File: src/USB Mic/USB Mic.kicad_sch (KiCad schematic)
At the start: 22 parts, among them IC1 ADUM3160BRWZ-RL, J1 GT-USB-7010ASV, Q1 LSK170B, U1 B0505S-3WR2_C7500927

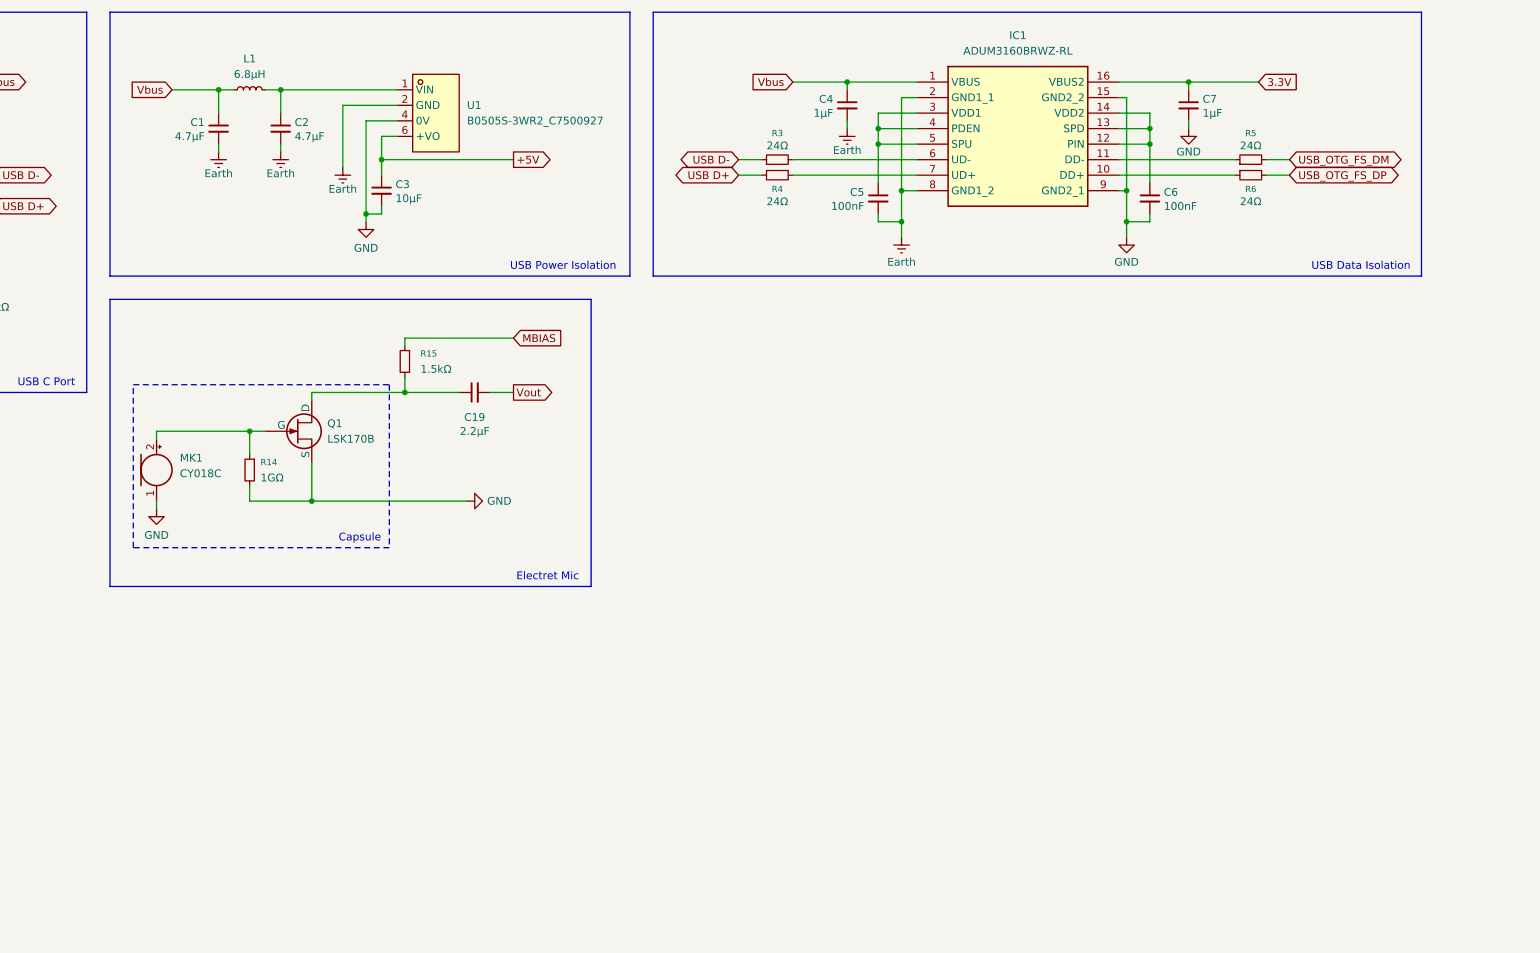
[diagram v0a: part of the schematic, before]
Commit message: Update to Rev. 5
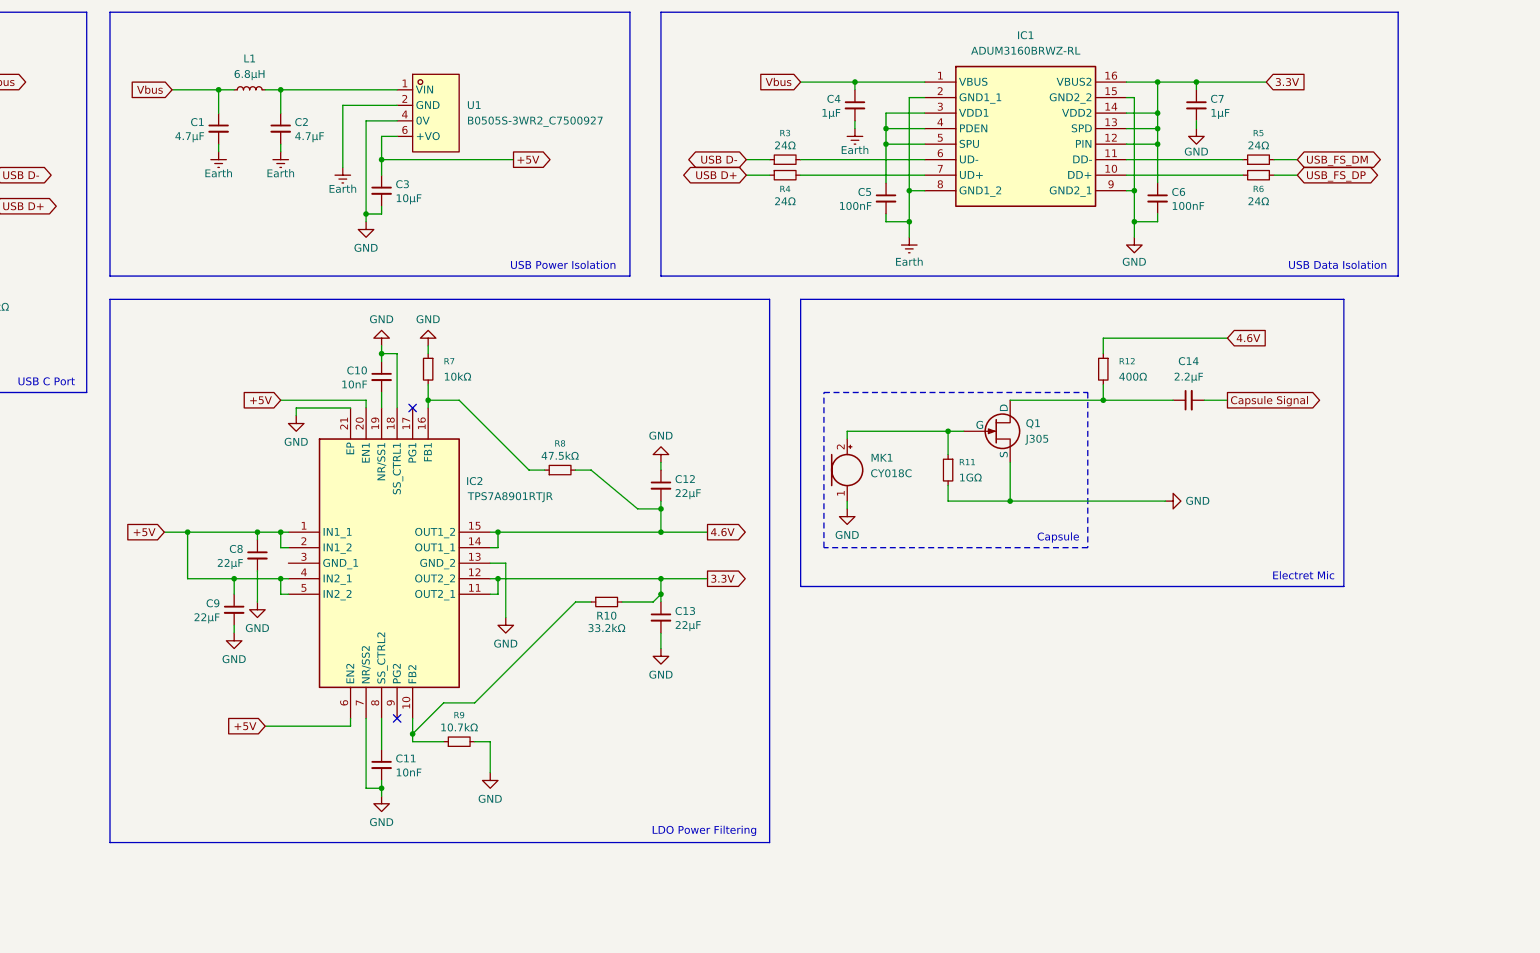
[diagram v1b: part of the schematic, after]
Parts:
- removed C19: 2.2µF, symbol Device:C_Small
- removed R14: 1GΩ, symbol Device:R_Small
- removed R15: 1.5kΩ, symbol Device:R_Small
- added C10, C11: 10nF, symbol Device:C_Small
- added C12, C13, C8, C9: 22µF, symbol Device:C_Small
- added C14: 2.2µF, symbol Device:C_Small
- added IC2: TPS7A8901RTJR, footprints:QFN50P400X400X80-21N-D, symbol TPS7A8901RTJR:TPS7A8901RTJR
- added R10: 33.2kΩ, symbol Device:R_Small
- added R11: 1GΩ, symbol Device:R_Small
- added R12: 400Ω, symbol Device:R_Small
- added R7: 10kΩ, symbol Device:R_Small
- added R8: 47.5kΩ, symbol Device:R_Small
- added R9: 10.7kΩ, symbol Device:R_Small
- Q1: value LSK170B -> J305
- U1: footprint easyeda2kicad:PWRM-TH_BXXXXS-3WR2 -> footprints:B0505S-3WR2
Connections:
- net +5V: now also C8.1, C9.1, IC2.1 (IN1_1), IC2.2 (IN1_2), IC2.20 (EN1), IC2.4 (IN2_1), IC2.5 (IN2_2), IC2.6 (EN2)
- net 3.3V: now also C6.1, IC1.12 (PIN), IC1.13 (SPD), IC1.14 (VDD2), C13.1, IC2.11 (OUT2_1), IC2.12 (OUT2_2), R10.2
- net GND: now also C10.1, C11.2, C12.1, C13.2, C8.2, C9.2, IC2.13 (GND_2), IC2.18 (SS_CTRL1), IC2.21 (EP), IC2.7 (NR/SS2), R11.2, R7.1, R9.2
- net at MK1.2 (+), Q1.2 (G): now also R11.1
- net at Q1.1 (D): now also C14.1, R12.2
- net USB_OTG_FS_DM renamed USB_FS_DM
- net USB_OTG_FS_DP renamed USB_FS_DP
- new net: IC2.10 (FB2), R10.1, R9.1
- new net: C10.2, IC2.19 (NR/SS1)
- new net: IC2.16 (FB1), R7.2, R8.1
- new net: C11.1, IC2.8 (SS_CTRL2)
- new net 4.6V: C12.2, IC2.14 (OUT1_1), IC2.15 (OUT1_2), R12.1, R8.2
- new net Capsule Signal: C14.2
- no-connect marks 2 -> 4
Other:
- note added: "LDO Power Filtering"
- moved on the sheet: C4, C5, C6, C7, IC1, MK1, Q1, R3, R4, R5, R6
